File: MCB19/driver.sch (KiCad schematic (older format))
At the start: 36 parts, among them J611 +BATT, J612 GND, J613 VBAT+, J614 VBAT-, Q601 IRFP260N, Q602 IRFP260N, U601 LM5104MNOPB, U602 INA211_DCK_6, U603 LM324

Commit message: New version
Detalhes
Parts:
- Q601, Q602: footprint KicadZeniteSolarLibrary18:TO-247-3_Horizontal_TabDown_SMD -> Package_TO_SOT_THT:TO-247-3_Vertical
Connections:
- net labels added: +15V
- wire segments 148 -> 147
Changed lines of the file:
@@
 $Descr A4 11693 8268
 encoding utf-8
-Sheet 6 6
+Sheet 6 7
 Title ""
 Date ""
@@
 $EndComp
 $Comp
-L power:+5V #PWR0605
-U 1 1 5D42E9E1
-P 2800 2700
-F 0 "#PWR0605" H 2800 2550 50  0001 C CNN
-F 1 "+5V" H 2815 2873 50  0000 C CNN
-F 2 "" H 2800 2700 50  0001 C CNN
-F 3 "" H 2800 2700 50  0001 C CNN
-	1    2800 2700
-	1    0    0    -1
-$EndComp
-$Comp
 L power:GND #PWR0606
 U 1 1 5D42EA3B
@@
 F 3 "" H 2800 2875 50  0001 C CNN
 	1    2800 2875
-	1    0    0    -1
-$EndComp
-Text HLabel 2850 2750 2    50   Input ~ 0
+	0    1    1    0
+$EndComp
+Text HLabel 2850 2700 2    50   Input ~ 0
 VCC
-Text HLabel 2850 2825 2    50   Input ~ 0
+Text HLabel 2850 2875 2    50   Input ~ 0
 GND
 Wire Wire Line
-	2850 2825 2800 2825
-Wire Wire Line
-	2800 2825 2800 2875
-Wire Wire Line
-	2850 2750 2800 2750
-Wire Wire Line
-	2800 2750 2800 2700
+	2850 2700 2800 2700
 $Comp
 L power:GND #PWR0604
@@
 Text HLabel 7250 2325 2    50   Output ~ 0
 IRALLL
-$Comp
-L power:+5V #PWR0109
-U 1 1 5D438678
-P 2250 2925
-F 0 "#PWR0109" H 2250 2775 50  0001 C CNN
-F 1 "+5V" H 2265 3098 50  0000 C CNN
-F 2 "" H 2250 2925 50  0001 C CNN
-F 3 "" H 2250 2925 50  0001 C CNN
-	1    2250 2925
-	1    0    0    -1
-$EndComp
 Wire Wire Line
 	2275 3900 2250 3900
@@
 F 0 "Q601" H 4900 2525 50  0000 L CNN
 F 1 "IRFP260N" H 4800 2450 50  0000 L CNN
-F 2 "KicadZeniteSolarLibrary18:TO-247-3_Horizontal_TabDown_SMD" H 5375 2425 50  0001 C CNN
+F 2 "Package_TO_SOT_THT:TO-247-3_Vertical" H 5375 2425 50  0001 C CNN
 F 3 "~" H 5175 2325 50  0001 C CNN
 	1    5175 2325
@@
 F 0 "Q602" H 4900 3175 50  0000 L CNN
 F 1 "IRFP260N" H 4775 3100 50  0000 L CNN
-F 2 "KicadZeniteSolarLibrary18:TO-247-3_Horizontal_TabDown_SMD" H 5375 3100 50  0001 C CNN
+F 2 "Package_TO_SOT_THT:TO-247-3_Vertical" H 5375 3100 50  0001 C CNN
 F 3 "~" H 5175 3000 50  0001 C CNN
 	1    5175 3000
@@
 Wire Wire Line
 	7650 2775 8425 2775
+$Comp
+L power:+5V #PWR0605
+U 1 1 5D42E9E1
+P 2800 2700
+F 0 "#PWR0605" H 2800 2550 50  0001 C CNN
+F 1 "+5V" H 2815 2873 50  0000 C CNN
+F 2 "" H 2800 2700 50  0001 C CNN
+F 3 "" H 2800 2700 50  0001 C CNN
+	1    2800 2700
+	0    -1   -1   0
+$EndComp
+Wire Wire Line
+	2800 2875 2850 2875
+Text HLabel 2850 2525 2    50   Input ~ 0
++15V
+$Comp
+L power:+15V #PWR0113
+U 1 1 5D9FF9B4
+P 2800 2525
+F 0 "#PWR0113" H 2800 2375 50  0001 C CNN
+F 1 "+15V" V 2815 2653 50  0000 L CNN
+F 2 "" H 2800 2525 50  0001 C CNN
+F 3 "" H 2800 2525 50  0001 C CNN
+	1    2800 2525
+	0    -1   -1   0
+$EndComp
+Wire Wire Line
+	2850 2525 2800 2525
+$Comp
+L power:+15V #PWR0114
+U 1 1 5DA059B9
+P 2250 2925
+F 0 "#PWR0114" H 2250 2775 50  0001 C CNN
+F 1 "+15V" H 2265 3098 50  0000 C CNN
+F 2 "" H 2250 2925 50  0001 C CNN
+F 3 "" H 2250 2925 50  0001 C CNN
+	1    2250 2925
+	1    0    0    -1
+$EndComp
 $EndSCHEMATC

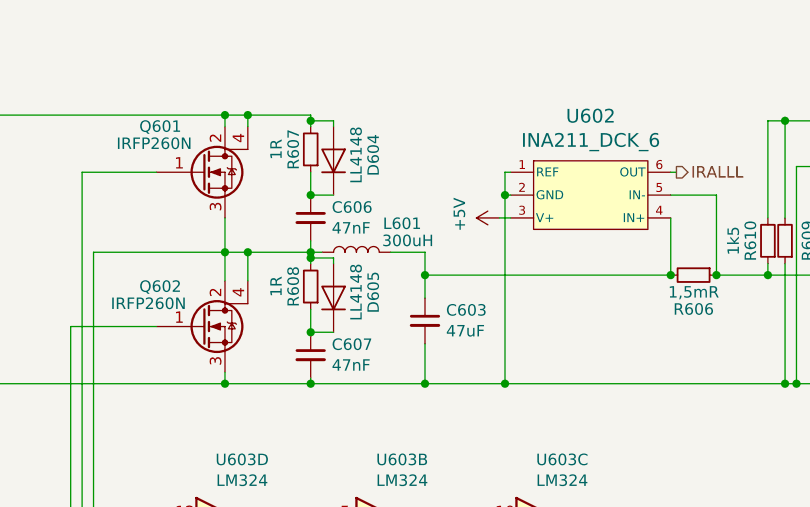
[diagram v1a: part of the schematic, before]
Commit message: Versão 2.0
Novas modificações, após confirmado, pode ser fabricada
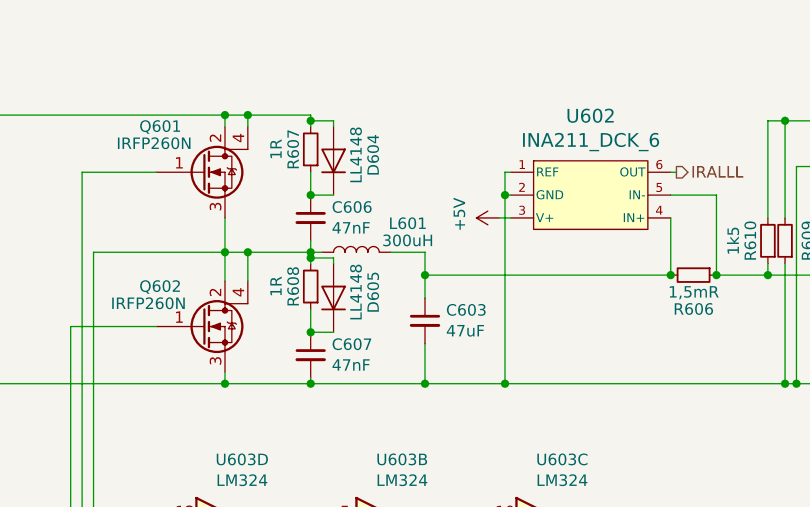
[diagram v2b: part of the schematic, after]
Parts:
- L601: footprint MCCplaca:Inductor_Nocoupled -> KicadZeniteSolarLibrary18:Inductor_Nocoupled
- Q601, Q602: footprint Package_TO_SOT_THT:TO-247-3_Vertical -> Package_TO_SOT_THT:TO-247-3_Horizontal_TabUp
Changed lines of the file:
@@
 F 0 "Q601" H 4900 2525 50  0000 L CNN
 F 1 "IRFP260N" H 4800 2450 50  0000 L CNN
-F 2 "Package_TO_SOT_THT:TO-247-3_Vertical" H 5375 2425 50  0001 C CNN
+F 2 "Package_TO_SOT_THT:TO-247-3_Horizontal_TabUp" H 5375 2425 50  0001 C CNN
 F 3 "~" H 5175 2325 50  0001 C CNN
 	1    5175 2325
@@
 F 0 "Q602" H 4900 3175 50  0000 L CNN
 F 1 "IRFP260N" H 4775 3100 50  0000 L CNN
-F 2 "Package_TO_SOT_THT:TO-247-3_Vertical" H 5375 3100 50  0001 C CNN
+F 2 "Package_TO_SOT_THT:TO-247-3_Horizontal_TabUp" H 5375 3100 50  0001 C CNN
 F 3 "~" H 5175 3000 50  0001 C CNN
 	1    5175 3000
@@
 U 1 1 5D42B749
 P 5850 2675
-F 0 "L601" V 5975 2475 50  0000 C CNN
+F 0 "L601" V 5975 2450 50  0000 C CNN
 F 1 "300uH" V 5900 2450 50  0000 C CNN
-F 2 "MCCplaca:Inductor_Nocoupled" H 5850 2675 50  0001 C CNN
+F 2 "KicadZeniteSolarLibrary18:Inductor_Nocoupled" H 5850 2675 50  0001 C CNN
 F 3 "~" H 5850 2675 50  0001 C CNN
 	1    5850 2675
